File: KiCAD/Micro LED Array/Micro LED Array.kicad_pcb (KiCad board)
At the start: 2 copper layers, 13 x 24.5 mm, 15 parts, among them J1 JST-XH

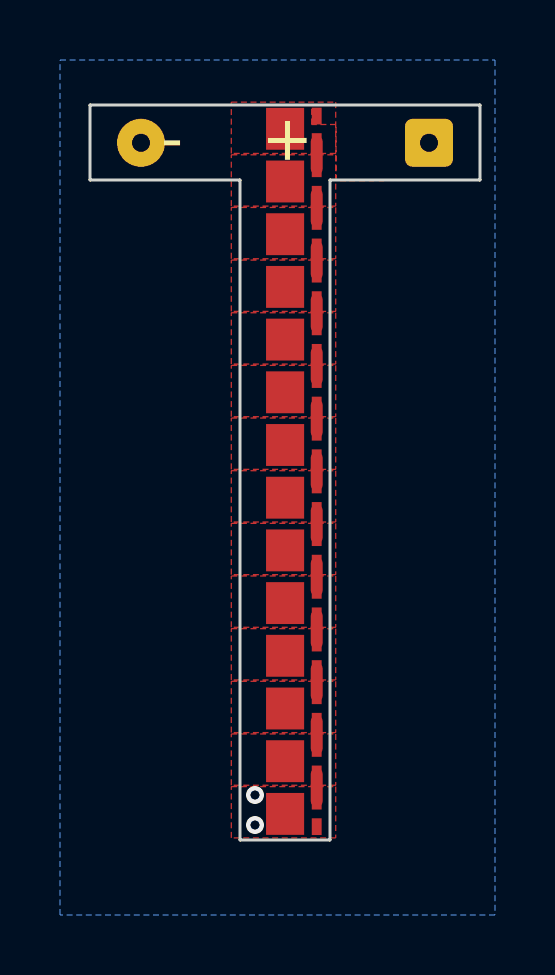
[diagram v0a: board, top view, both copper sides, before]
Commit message: Ordered version
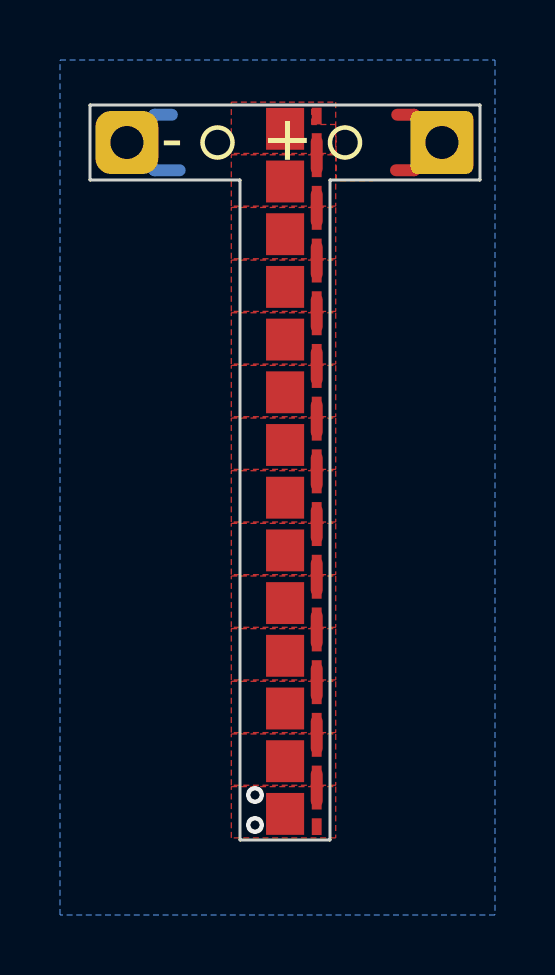
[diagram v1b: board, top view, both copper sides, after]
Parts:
- J1: footprint Custom footprints:SolderWire-0.1sqmm_1x02_P9.6mm_D0.4mm_OD1mm -> Custom footprints:SolderWire-0.5sqmm_1x02_P10.5mm_D0.9mm_OD2.1mm
- moved J1 0.43 mm to (36.7, 25.2)
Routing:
- net VSS: track 0.00 -> 4.03 mm
- net VDD: track 0.00 -> 3.79 mm
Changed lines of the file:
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@@
     )
   )
-  (footprint "Custom footprints:SolderWire-0.1sqmm_1x02_P9.6mm_D0.4mm_OD1mm" (layer "F.Cu")
-    (at 36.3 25.26 180)
-    (descr "Soldered wire connection, for 2 times 0.1 mm² wires, basic insulation, conductor diameter 0.4mm, outer diameter 1mm, size source Multi-Contact FLEXI-E 0.1 (https://ec.staubli.com/AcroFiles/Catalogues/TM_Cab-Main-11014119_(en)_hi.pdf), bend radius 3 times outer diameter, generated with kicad-footprint-generator")
-    (tags "connector wire 0.1sqmm")
+  (footprint "Custom footprints:SolderWire-0.5sqmm_1x02_P10.5mm_D0.9mm_OD2.1mm" (layer "F.Cu")
+    (at 36.73 25.25 180)
+    (descr "Soldered wire connection, for 2 times 0.5 mm² wires, basic insulation, conductor diameter 0.9mm, outer diameter 2.1mm, size source Multi-Contact FLEXI-E 0.5 (https://ec.staubli.com/AcroFiles/Catalogues/TM_Cab-Main-11014119_(en)_hi.pdf), bend radius 3 times outer diameter, generated with kicad-footprint-generator")
+    (tags "connector wire 0.5sqmm")
     (property "Manufacturer" "JST Sales America Inc.")
     (property "Part" "B2B-XH-A")
@@
     (property "ki_description" "Generic connector, single row, 01x02, script generated")
     (property "ki_keywords" "connector")
-    (clearance 2.5)
     (zone_connect 1)
     (attr exclude_from_pos_files)
-    (fp_text reference "J1" (at 6.72 -0.21) (layer "F.SilkS") hide
-        (effects (font (size 1 1) (thickness 0.15)))
-    )
-    (fp_text value "JST-XH" (at 3.8 2) (layer "F.Fab") hide
-        (effects (font (size 1 1) (thickness 0.15)))
-    )
-    (fp_line (start -1.3 -1.3) (end -1.3 1.3)
-      (stroke (width 0.05) (type solid)) (layer "F.CrtYd"))
-    (fp_line (start -1.3 1.3) (end 1.3 1.3)
-      (stroke (width 0.05) (type solid)) (layer "F.CrtYd"))
-    (fp_line (start 1.3 -1.3) (end -1.3 -1.3)
-      (stroke (width 0.05) (type solid)) (layer "F.CrtYd"))
-    (fp_line (start 1.3 1.3) (end 1.3 -1.3)
-      (stroke (width 0.05) (type solid)) (layer "F.CrtYd"))
-    (fp_line (start 8.3 -1.3) (end 8.3 1.3)
-      (stroke (width 0.05) (type solid)) (layer "F.CrtYd"))
-    (fp_line (start 8.3 1.3) (end 10.9 1.3)
-      (stroke (width 0.05) (type solid)) (layer "F.CrtYd"))
-    (fp_line (start 10.9 -1.3) (end 8.3 -1.3)
-      (stroke (width 0.05) (type solid)) (layer "F.CrtYd"))
-    (fp_line (start 10.9 1.3) (end 10.9 -1.3)
-      (stroke (width 0.05) (type solid)) (layer "F.CrtYd"))
-    (fp_circle (center 0 0) (end 0.5 0)
+    (fp_text reference "J1" (at 7.18 1.89 180) (layer "F.SilkS") hide
+        (effects (font (size 1 1) (thickness 0.15)))
+    )
+    (fp_text value "JST-XH" (at 2.3 2.25 180) (layer "F.Fab") hide
+        (effects (font (size 1 1) (thickness 0.15)))
+    )
+    (fp_line (start -1.8 -1.55) (end -1.8 1.55)
+      (stroke (width 0.05) (type solid)) (layer "F.CrtYd"))
+    (fp_line (start -1.8 1.55) (end 1.8 1.55)
+      (stroke (width 0.05) (type solid)) (layer "F.CrtYd"))
+    (fp_line (start 1.8 -1.55) (end -1.8 -1.55)
+      (stroke (width 0.05) (type solid)) (layer "F.CrtYd"))
+    (fp_line (start 1.8 1.55) (end 1.8 -1.55)
+      (stroke (width 0.05) (type solid)) (layer "F.CrtYd"))
+    (fp_line (start 8.7 -1.55) (end 8.7 1.55)
+      (stroke (width 0.05) (type solid)) (layer "F.CrtYd"))
+    (fp_line (start 8.7 1.55) (end 12.3 1.55)
+      (stroke (width 0.05) (type solid)) (layer "F.CrtYd"))
+    (fp_line (start 12.3 -1.55) (end 8.7 -1.55)
+      (stroke (width 0.05) (type solid)) (layer "F.CrtYd"))
+    (fp_line (start 12.3 1.55) (end 12.3 -1.55)
+      (stroke (width 0.05) (type solid)) (layer "F.CrtYd"))
+    (fp_circle (center 0 0) (end 1.05 0)
       (stroke (width 0.1) (type solid)) (fill none) (layer "F.Fab"))
-    (fp_circle (center 9.6 0) (end 10.1 0)
+    (fp_circle (center 10.5 0) (end 11.55 0)
       (stroke (width 0.1) (type solid)) (fill none) (layer "F.Fab"))
-    (pad "1" thru_hole roundrect (at 0 0 180) (size 1.6 1.6) (drill 0.6) (layers "*.Cu" "*.Mask") (roundrect_rratio 0.15625)
-      (net 1 "VDD") (pinfunction "Pin_1") (pintype "passive") (thermal_bridge_width 0.5) (thermal_bridge_angle 45))
-    (pad "2" thru_hole circle (at 9.6 0 180) (size 1.6 1.6) (drill 0.6) (layers "*.Cu" "*.Mask")
-      (net 11 "VSS") (pinfunction "Pin_2") (pintype "passive"))
-    (model "${KICAD6_3DMODEL_DIR}/Connector_Wire.3dshapes/SolderWire-0.1sqmm_1x02_P3.6mm_D0.4mm_OD1mm.wrl"
+    (pad "1" thru_hole roundrect (at 0 0 180) (size 2.1 2.1) (drill 1.1) (layers "*.Cu" "*.Mask") (roundrect_rratio 0.1190480952)
+      (net 1 "VDD") (pinfunction "Pin_1") (pintype "passive") (clearance 3) (thermal_bridge_width 0.4) (thermal_bridge_angle 45) (thermal_gap 0.3))
+    (pad "2" thru_hole roundrect (at 10.5 0 180) (size 2.1 2.1) (drill 1.1) (layers "*.Cu" "*.Mask") (roundrect_rratio 0.25)
+      (net 11 "VSS") (pinfunction "Pin_2") (pintype "passive") (clearance 3) (thermal_bridge_width 0.4) (thermal_bridge_angle 45) (thermal_gap 0.3))
+    (model "${KICAD6_3DMODEL_DIR}/Connector_Wire.3dshapes/SolderWire-0.5sqmm_1x02_P4.6mm_D0.9mm_OD2.1mm.wrl"
       (offset (xyz 0 0 0))
       (scale (xyz 1 1 1))
@@
     )
   )
+  (gr_circle (center 29.25 25.25) (end 29.75 25.25)
+    (stroke (width 0.15) (type default)) (fill none) (layer "F.SilkS"))
+  (gr_circle (center 33.5 25.25) (end 34 25.25)
+    (stroke (width 0.15) (type default)) (fill none) (layer "F.SilkS"))
   (gr_line (start 38 26.5) (end 38 24)
     (stroke (width 0.1) (type default)) (layer "Edge.Cuts"))
@@
     (effects (font (size 1.5 1.5) (thickness 0.15)) (justify left bottom))
   )
+  (segment (start 36.73 25.25) (end 35.805 24.325) (width 0.4) (layer "F.Cu") (net 1))
+  (segment (start 35.805 26.175) (end 35.2 26.175) (width 0.4) (layer "F.Cu") (net 1))
+  (segment (start 36.73 25.25) (end 35.805 26.175) (width 0.4) (layer "F.Cu") (net 1))
+  (segment (start 35.805 24.325) (end 35.24 24.325) (width 0.4) (layer "F.Cu") (net 1))
   (segment (start 32.557 39.27167) (end 32.557 40.178336) (width 0.4) (layer "F.Cu") (net 2))
   (segment (start 32.557 41.028336) (end 32.557 41.935002) (width 0.4) (layer "F.Cu") (net 3))
@@
   (via (at 30.5 48) (size 0.6) (drill 0.3) (layers "F.Cu" "B.Cu") (free) (net 11))
   (via (at 30.5 47) (size 0.6) (drill 0.3) (layers "F.Cu" "B.Cu") (free) (net 11))
+  (segment (start 27.155 26.175) (end 27.99 26.175) (width 0.4) (layer "B.Cu") (net 11))
+  (segment (start 27.155 24.325) (end 27.73 24.325) (width 0.4) (layer "B.Cu") (net 11))
+  (segment (start 26.23 25.25) (end 27.155 24.325) (width 0.4) (layer "B.Cu") (net 11))
+  (segment (start 26.23 25.25) (end 27.155 26.175) (width 0.4) (layer "B.Cu") (net 11))
   (segment (start 32.557 34.001672) (end 32.557 34.908338) (width 0.4) (layer "F.Cu") (net 12))
   (segment (start 32.557 35.758338) (end 32.557 36.665004) (width 0.4) (layer "F.Cu") (net 13))
